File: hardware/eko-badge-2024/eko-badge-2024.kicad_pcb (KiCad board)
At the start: 2 copper layers, 47.5 x 99.9 mm, 2 parts

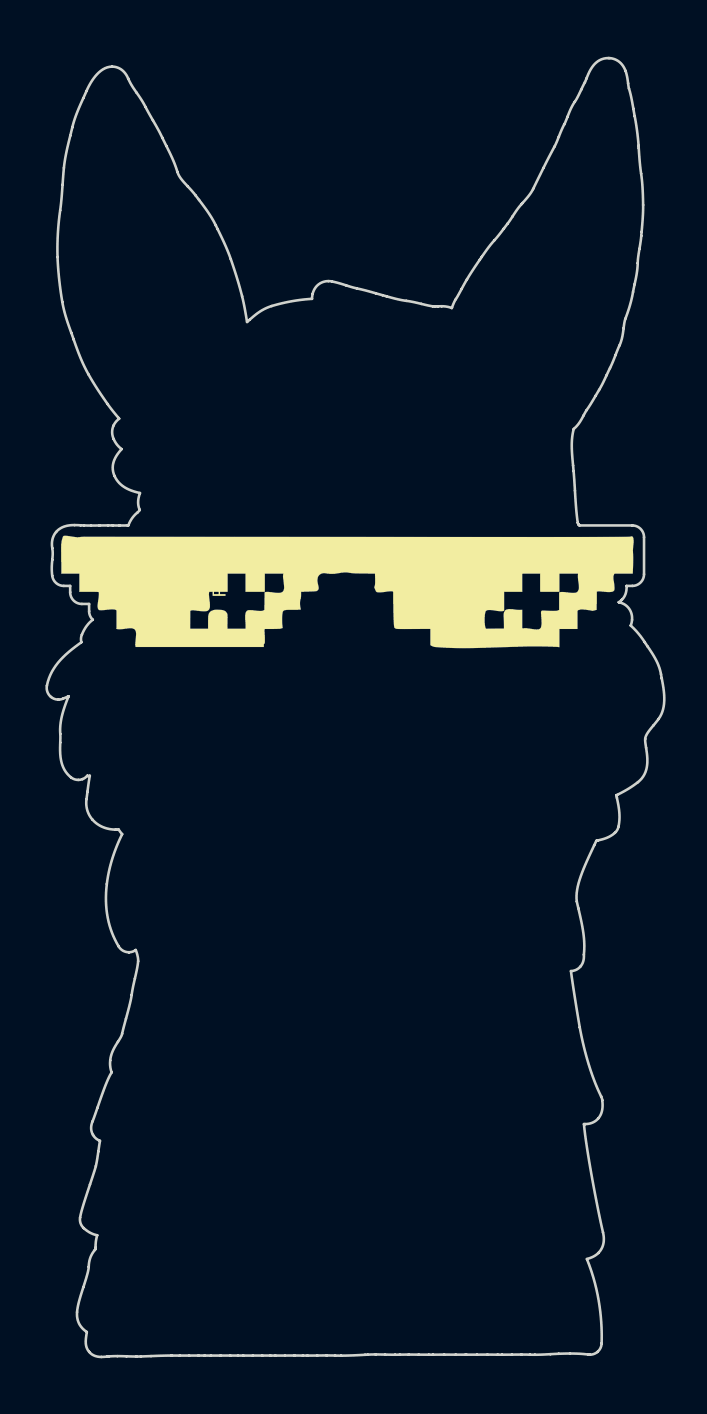
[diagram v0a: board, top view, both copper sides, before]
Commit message: feat(Hw):Added_First_Route
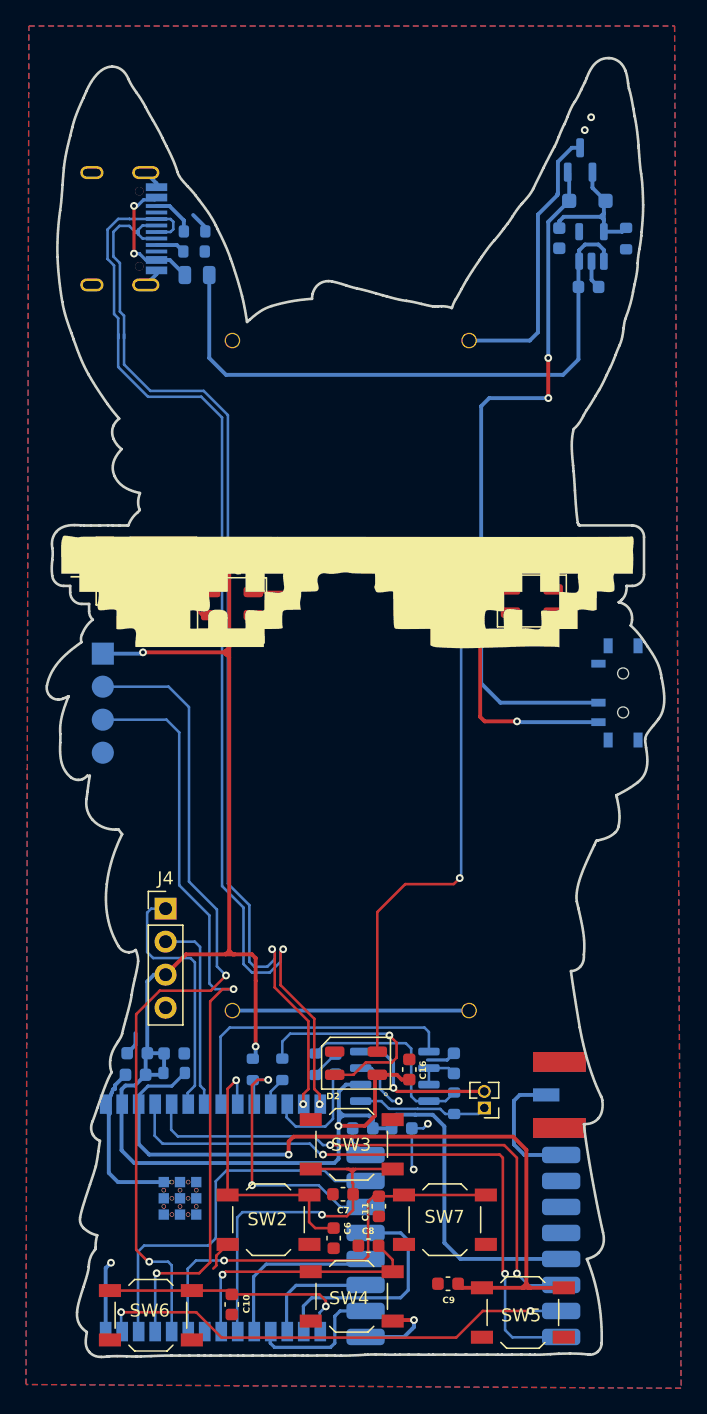
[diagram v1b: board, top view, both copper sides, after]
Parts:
- removed REF**: PinSocket_2x03_P2.54mm_Vertical, Connector_PinSocket_2.54mm:PinSocket_2x03_P2.54mm_Vertical
- added AE1: Antenna_Shield, Eko2024:SMA_EDGE, B.Cu at (221.3, 109.9)
- added C1: 10uF, Capacitor_SMD:C_0603_1608Metric, B.Cu at (221.5, 47.7)
- added C10: .1uF, Capacitor_SMD:C_0603_1608Metric, F.Cu at (194.1, 126.0)
- added C11: .1uF, Capacitor_SMD:C_0603_1608Metric, F.Cu at (205.4, 118.5)
- added C12: 0.1uF, Capacitor_SMD:C_0603_1608Metric, B.Cu at (204.2, 112.5)
- added C13: .22uF, Capacitor_SMD:C_0603_1608Metric, B.Cu at (202.1, 107.5)
- added C14: .1uF, Capacitor_SMD:C_0603_1608Metric, B.Cu at (211.2, 107.5)
- added C15: 1uF, Capacitor_SMD:C_0603_1608Metric, B.Cu at (207.2, 112.5)
- added C16: 0.1uF, Capacitor_SMD:C_0603_1608Metric, F.Cu at (207.7, 107.9)
- added C17: 0.1uF, Capacitor_SMD:C_0603_1608Metric, F.Cu at (194.6, 69.3)
- added C18: 0.1uF, Capacitor_SMD:C_0603_1608Metric, F.Cu at (216.1, 69.1)
- added C2: 1uF, Capacitor_SMD:C_0603_1608Metric, B.Cu at (189.6, 106.7)
- added C3: 10uF, Capacitor_SMD:C_0603_1608Metric, B.Cu at (219.3, 44.0)
- added C4: 10uF, Capacitor_SMD:C_0603_1608Metric, B.Cu at (186.8, 106.7)
- added C5: 10uF, Capacitor_SMD:C_0603_1608Metric, B.Cu at (186.7, 108.3)
- added C6: .1uF, Capacitor_SMD:C_0603_1608Metric, F.Cu at (201.9, 120.9)
- added C7: .1uF, Capacitor_SMD:C_0603_1608Metric, F.Cu at (202.6, 117.5)
- added C8: .1uF, Capacitor_SMD:C_0603_1608Metric, F.Cu at (204.6, 121.5)
- added C9: .1uF, Capacitor_SMD:C_0603_1608Metric, F.Cu at (210.7, 124.4)
- added D1: MBR120, Diode_SMD:D_SOD-123F, B.Cu at (221.4, 41.1)
- added D2: WS2812B, LED_SMD:LED_WS2812B-Mini_PLCC4_3.5x3.5mm, F.Cu at (203.6, 107.5)
- added D3: WS2812B, LED_SMD:LED_WS2812B-Mini_PLCC4_3.5x3.5mm, F.Cu at (194.1, 72.1)
- added D4: WS2812B, LED_SMD:LED_WS2812B-Mini_PLCC4_3.5x3.5mm, F.Cu at (217.2, 71.9)
- added F1: 0.75A, Fuse:Fuse_0805_2012Metric, B.Cu at (191.4, 46.8)
- added J1: UART, Connector_PinHeader_2.54mm:PinHeader_1x04_P2.54mm_Vertical, B.Cu at (184.2, 76.0)
- added J2: Battery, Eko2024:BH-AA-A1AJ020, B.Cu at (212.3, 77.6)
- added J3: Lentes, Connector_PinSocket_2.54mm:PinSocket_2x03_P2.54mm_Vertical, F.Cu at (185.0, 68.3)
- added J4: OLED, Eko2024:Display OLED 128 x32, F.Cu at (189.0, 95.6)
- added J7: Battery, Eko2024:BH-AA-A1AJ020, B.Cu at (194.1, 77.6)
- added LS1: 931-SPKM.20.8.A-ND, Connector_PinHeader_1.27mm:PinHeader_1x02_P1.27mm_Vertical, F.Cu at (213.5, 110.9)
- added P1: USB_C_Plug_USB2.0, Eko2024:C393939, B.Cu at (187.5, 43.3)
- added Q1: DMG3415U-7, Package_TO_SOT_SMD:SOT-23, B.Cu at (220.9, 38.0)
- added R1: 100K, Resistor_SMD:R_0603_1608Metric, B.Cu at (224.4, 44.0)
- added R2: 10K, Resistor_SMD:R_0603_1608Metric, B.Cu at (189.6, 108.2)
- added R3: 5k1, Resistor_SMD:R_0603_1608Metric, B.Cu at (191.2, 45.0)
- added R4: 5k1, Resistor_SMD:R_0603_1608Metric, B.Cu at (191.2, 43.5)
- added R5: 47K, Resistor_SMD:R_0603_1608Metric, B.Cu at (200.5, 107.5)
- added R6: 22K, Resistor_SMD:R_0603_1608Metric, B.Cu at (211.2, 110.5)
- added R7: 470, Resistor_SMD:R_0603_1608Metric, B.Cu at (198.0, 107.9)
- added R8: 3.3K, Resistor_SMD:R_0603_1608Metric, B.Cu at (195.7, 107.9)
- added SW1: ON, Eko2024:MSK12C02, B.Cu at (224.2, 79.0)
- added SW2: LEFT, Button_Switch_SMD:SW_SPST_TL3342, F.Cu at (196.9, 119.5)
- added SW3: UP, Button_Switch_SMD:SW_SPST_TL3342, F.Cu at (203.3, 113.7)
- added SW4: DOWN, Button_Switch_SMD:SW_SPST_TL3342, F.Cu at (203.3, 125.4)
- added SW5: RESET, Button_Switch_SMD:SW_SPST_TL3342, F.Cu at (216.5, 126.6)
- added SW6: BOOT, Button_Switch_SMD:SW_SPST_TL3342, F.Cu at (187.8, 126.8)
- added SW7: RIGTH, Button_Switch_SMD:SW_SPST_TL3342, F.Cu at (210.5, 119.5)
- added U1: ESP32-C6-WROOM-1-N4, bsides:XCVR_ESP32-C6-WROOM-1-N8, B.Cu at (189.6, 119.4)
- added U2: AP2112K-3.3, Package_TO_SOT_SMD:SOT-23-5, B.Cu at (221.8, 44.6)
- added U3: RFM95W-868S2, RF_Module:HOPERF_RFM9XW_SMD, B.Cu at (211.9, 121.5)
- added U4: TPA321, Package_SO:SOP-8_3.9x4.9mm_P1.27mm, B.Cu at (206.6, 108.5)
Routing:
- net /VOUT: track 0.00 -> 190.5 mm, vias 0 -> 4
- net /D+: track 0.00 -> 88.8 mm, vias 0 -> 2
- net /D-: track 0.00 -> 86.0 mm, vias 0 -> 2
- net /RX: track 0.00 -> 63.7 mm, vias 0 -> 2
- net /EN: track 0.00 -> 60.0 mm, vias 0 -> 1
- net /TX: track 0.00 -> 59.9 mm, vias 0 -> 2
- net Net-(D2-DOUT): track 0.00 -> 59.2 mm, vias 0 -> 2
- net Net-(D1-K): track 0.00 -> 54.5 mm, vias 0 -> 2
- net GND: track 0.00 -> 50.5 mm, vias 0 -> 7
- net /DIO2: track 0.00 -> 47.8 mm, vias 0 -> 2
- net VBUS: track 0.00 -> 47.4 mm
- net /DIO0: track 0.00 -> 42.2 mm, vias 0 -> 2
- net Net-(D3-DOUT): track 0.00 -> 37.5 mm
- net /DIO1: track 0.00 -> 37.4 mm, vias 0 -> 2
- net /RIGHT: track 0.00 -> 32.6 mm, vias 0 -> 1
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- added copper zone on B.Cu, net GND
- added copper zone on F.Cu, net GND
